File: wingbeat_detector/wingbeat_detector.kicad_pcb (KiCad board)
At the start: 4 copper layers, 32 x 18 mm, 38 parts, among them J1 USB_C_10137062-00021LF, J2 UMC_JACK_SMD, J3 UMC_JACK_SMD, U1 MAX865EUA+, U2 UAF42_SMA, U3 UAF42_SMA, U4 OPA381

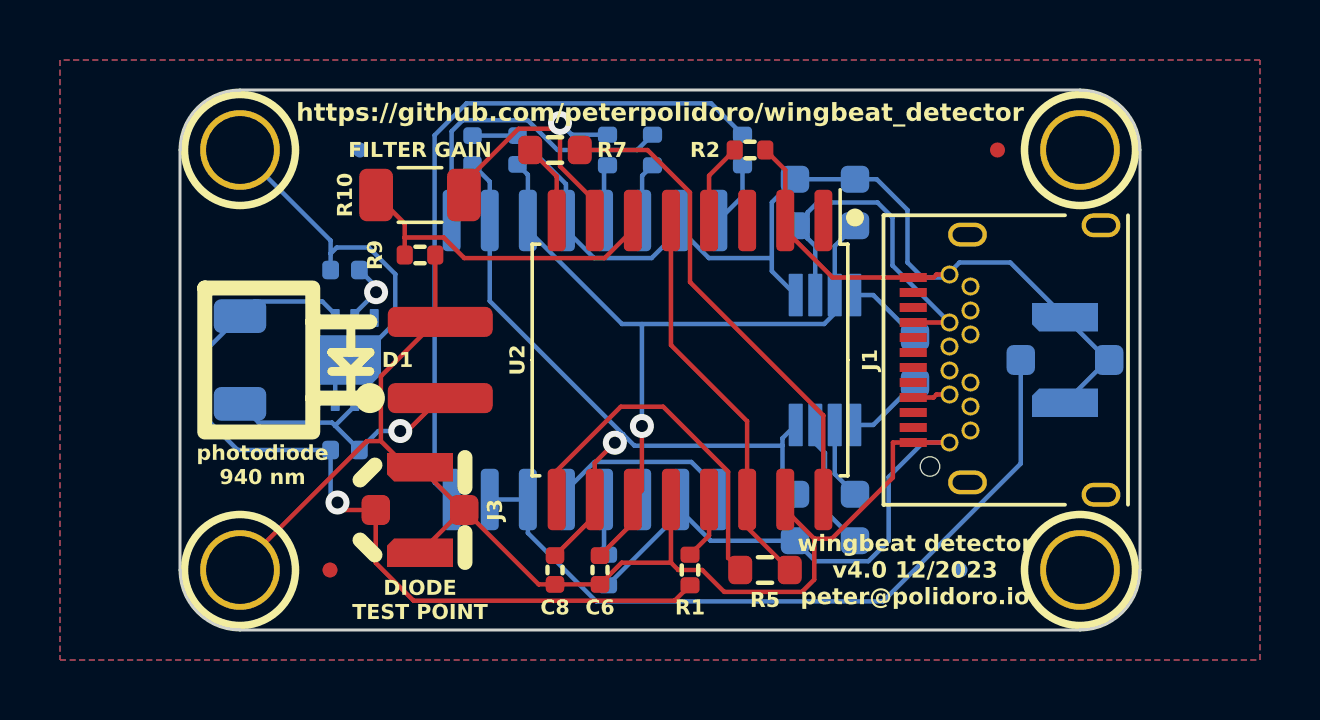
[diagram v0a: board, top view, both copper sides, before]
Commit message: Update images and documentation
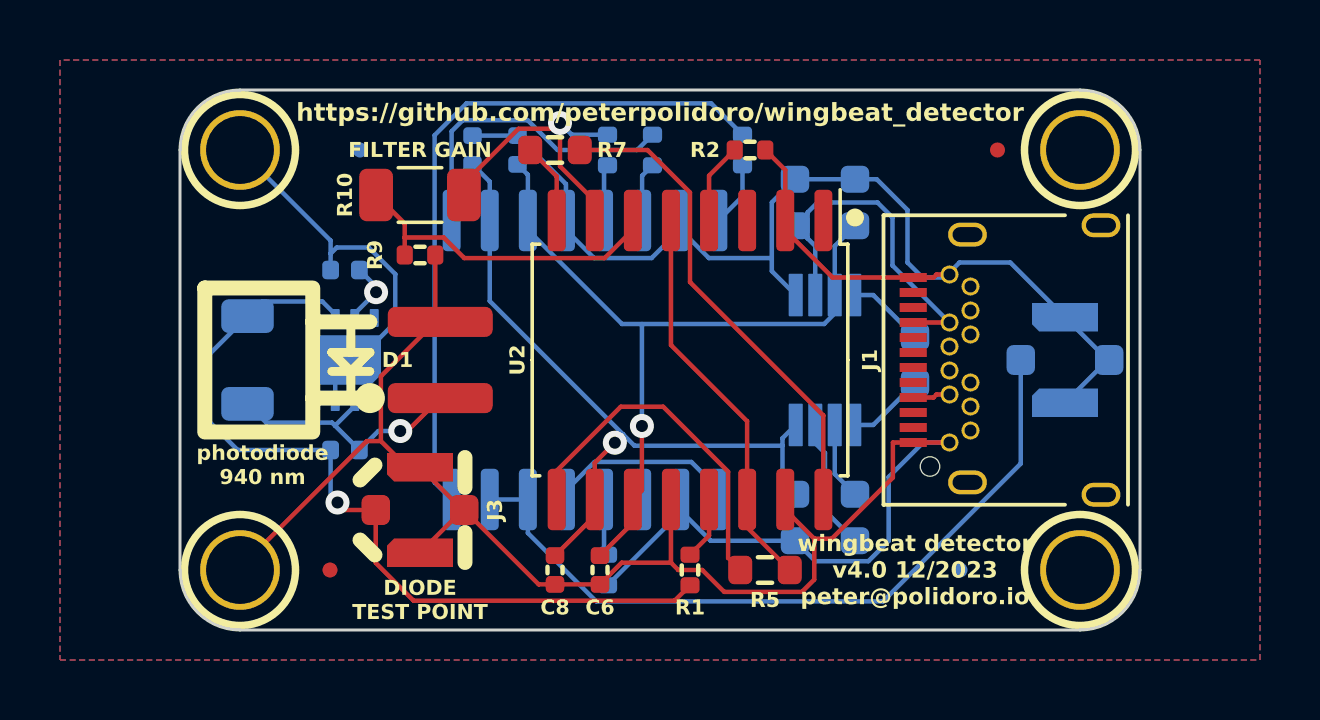
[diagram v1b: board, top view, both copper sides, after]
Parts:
- R10: value GAIN1 -> 150k
- moved R11 0.25 mm to (136.2, 100.0)
